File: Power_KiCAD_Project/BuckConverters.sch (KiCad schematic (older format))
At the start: 14 parts

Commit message: added components
added a few components and the correct numbers
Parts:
- removed D? (x2): SBRD10200TR, symbol Device:D_Schottky
- added D5, D6: SBRD10200TR, SBRD10200TR:DPAK228P1005X240-4N, symbol SBRD10200TR:SBRD10200TR
- C21, C22: renamed from C?; symbol 35SVPF82M:35SVPF82M -> Power_KiCAD_Project-rescue:35SVPF82M-35SVPF82M
- C27: renamed from C?; symbol 16SVP330M:16SVP330M -> Power_KiCAD_Project-rescue:16SVP330M-16SVP330M
- C28: renamed from C?; symbol 6SVPC330M:6SVPC330M -> Power_KiCAD_Project-rescue:6SVPC330M-6SVPC330M
- U5, U6: renamed from U?; symbol lm2672m-to-263:LM2672M-TO-263 -> Power_KiCAD_Project-rescue:LM2672M-TO-263-lm2672m-to-263
- gave numbers to parts that had none: 6
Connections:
- net labels added: ground
- net labels removed: GND
- wire segments 46 -> 50
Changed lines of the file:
@@
 $Descr A4 11693 8268
 encoding utf-8
-Sheet 12 12
+Sheet 6 12
 Title "Buck Converter Supply"
 Date "2021-11-29"
@@
 $EndDescr
 $Comp
-L lm2672m-to-263:LM2672M-TO-263 U?
+L Power_KiCAD_Project-rescue:LM2672M-TO-263-lm2672m-to-263 U6
 U 1 1 61A319C7
 P 4900 5200
-F 0 "U?" H 4900 5667 50  0000 C CNN
+F 0 "U6" H 4900 5667 50  0000 C CNN
 F 1 "LM2678SX-3.3/NOPB" H 4900 5576 50  0000 C CNN
 F 2 "Package_TO_SOT_SMD:TO-263-7_TabPin8" H 4950 4850 50  0001 L CIN
@@
 $EndComp
 $Comp
-L Device:C C?
+L Device:C C24
 U 1 1 61A53C7C
 P 4050 5400
-F 0 "C?" H 4200 5400 50  0000 L CNN
+F 0 "C24" H 4200 5400 50  0000 L CNN
 F 1 "C0805C104M5RACTU" V 3900 5000 50  0000 L CNN
 F 2 "Capacitor_SMD:C_0805_2012Metric" H 4088 5250 50  0001 C CNN
@@
 Designed with 3S - 5S lithium pack in mind\nV_IN: 9V - 21V\n\n5A Output
 $Comp
-L 35SVPF82M:35SVPF82M C?
+L Power_KiCAD_Project-rescue:35SVPF82M-35SVPF82M C22
 U 1 1 61A4499B
 P 3400 5250
-F 0 "C?" V 3550 5350 60  0000 L CNN
+F 0 "C22" V 3550 5350 60  0000 L CNN
 F 1 "35SVPF82M" H 3350 5100 60  0000 L CNN
 F 2 "35SVPF82M:35SVPF82M" H 3550 4890 60  0001 C CNN
@@
 	4050 5000 4400 5000
 $Comp
-L Device:C_Small C?
+L Device:C_Small C26
 U 1 1 61A48396
 P 5650 5300
-F 0 "C?" H 5742 5346 50  0000 L CNN
+F 0 "C26" H 5742 5346 50  0000 L CNN
 F 1 "CGA4C2C0G1H103J060AA" H 5700 5250 39  0000 L CNN
 F 2 "Capacitor_SMD:C_0805_2012Metric" H 5650 5300 50  0001 C CNN
@@
 $EndComp
 $Comp
-L pspice:INDUCTOR L?
+L pspice:INDUCTOR L2
 U 1 1 61A496D2
 P 6950 5400
-F 0 "L?" H 6950 5615 50  0000 C CNN
+F 0 "L2" H 6950 5615 50  0000 C CNN
 F 1 "SER2915L-103KL" H 6950 5524 50  0000 C CNN
 F 2 "SER2915L-153KL:SER2915L-153KL" H 6950 5400 50  0001 C CNN
@@
 $EndComp
 $Comp
-L 6SVPC330M:6SVPC330M C?
+L Power_KiCAD_Project-rescue:6SVPC330M-6SVPC330M C28
 U 1 1 61A467E9
 P 7400 5550
-F 0 "C?" V 7500 5750 60  0000 L CNN
+F 0 "C28" V 7500 5750 60  0000 L CNN
 F 1 "6SVPC330M" H 7300 5700 60  0000 L CNN
 F 2 "6SVPC330M:6SVPC330M" H 7550 5190 60  0001 C CNN
@@
 Wire Wire Line
 	7200 5400 7400 5400
-$Comp
-L Device:D_Schottky D?
-U 1 1 61A4C464
-P 6100 5700
-F 0 "D?" V 6054 5780 50  0000 L CNN
-F 1 "SBRD10200TR" H 5850 5600 50  0000 L CNN
-F 2 "" H 6100 5700 50  0001 C CNN
-F 3 "~" H 6100 5700 50  0001 C CNN
-	1    6100 5700
-	0    1    1    0
-$EndComp
-Wire Wire Line
-	6100 6000 6100 5850
-Wire Wire Line
-	6100 6000 7400 6000
-Wire Wire Line
-	6100 5550 6100 5400
-Wire Wire Line
-	6100 5400 6700 5400
+Wire Wire Line
+	6100 6000 6300 6000
 Wire Wire Line
 	7400 5850 7400 6000
@@
 Wire Wire Line
 	5400 5200 5650 5200
-Wire Wire Line
-	5650 5400 6100 5400
 Connection ~ 5650 5400
-Connection ~ 6100 5400
 Wire Wire Line
 	7400 5000 7400 5400
 Wire Wire Line
 	5400 5000 7400 5000
-Connection ~ 6100 6000
-$Comp
-L power:GND #PWR?
-U 1 1 61A58607
-P 4050 5800
-F 0 "#PWR?" H 4050 5550 50  0001 C CNN
-F 1 "GND" H 4055 5627 50  0000 C CNN
-F 2 "" H 4050 5800 50  0001 C CNN
-F 3 "" H 4050 5800 50  0001 C CNN
-	1    4050 5800
-	1    0    0    -1
-$EndComp
-$Comp
-L power:GND #PWR?
-U 1 1 61A58BE6
-P 6100 6000
-F 0 "#PWR?" H 6100 5750 50  0001 C CNN
-F 1 "GND" H 6105 5827 50  0000 C CNN
-F 2 "" H 6100 6000 50  0001 C CNN
-F 3 "" H 6100 6000 50  0001 C CNN
-	1    6100 6000
-	1    0    0    -1
-$EndComp
 NoConn ~ 4400 5400
 Wire Notes Line
@@
 3.3V Buck Converter
 $Comp
-L lm2672m-to-263:LM2672M-TO-263 U?
+L Power_KiCAD_Project-rescue:LM2672M-TO-263-lm2672m-to-263 U5
 U 1 1 61A7F0DE
 P 4900 2850
-F 0 "U?" H 4900 3317 50  0000 C CNN
+F 0 "U5" H 4900 3317 50  0000 C CNN
 F 1 "LM2678SX-5.0/NOPB" H 4900 3226 50  0000 C CNN
 F 2 "Package_TO_SOT_SMD:TO-263-7_TabPin8" H 4950 2500 50  0001 L CIN
@@
 $EndComp
 $Comp
-L Device:C C?
+L Device:C C23
 U 1 1 61A7F0E5
 P 4050 3050
-F 0 "C?" H 4200 3050 50  0000 L CNN
+F 0 "C23" H 4200 3050 50  0000 L CNN
 F 1 "C0805C104M5RACTU" V 3900 2650 50  0000 L CNN
 F 2 "Capacitor_SMD:C_0805_2012Metric" H 4088 2900 50  0001 C CNN
@@
 $EndComp
 Wire Wire Line
-	3400 2650 3400 2900
-Wire Wire Line
 	3400 3450 3400 3200
 Wire Wire Line
 	4900 3450 4900 3250
-Wire Wire Line
-	3400 2650 3250 2650
-Connection ~ 3400 2650
 Text HLabel 3250 2650 0    50   Input ~ 0
 V_IN
 $Comp
-L 35SVPF82M:35SVPF82M C?
+L Power_KiCAD_Project-rescue:35SVPF82M-35SVPF82M C21
 U 1 1 61A7F0F2
 P 3400 2900
-F 0 "C?" V 3550 3000 60  0000 L CNN
+F 0 "C21" V 3550 3000 60  0000 L CNN
 F 1 "35SVPF82M" H 3350 2750 60  0000 L CNN
 F 2 "35SVPF82M:35SVPF82M" H 3550 2540 60  0001 C CNN
@@
 	3400 3450 4050 3450
 Wire Wire Line
-	3400 2650 4050 2650
-Wire Wire Line
 	4050 3200 4050 3450
 Connection ~ 4050 3450
@@
 	4050 2650 4400 2650
 $Comp
-L Device:C_Small C?
+L Device:C_Small C25
 U 1 1 61A7F101
 P 5650 2950
-F 0 "C?" H 5742 2996 50  0000 L CNN
+F 0 "C25" H 5742 2996 50  0000 L CNN
 F 1 "CGA4C2C0G1H103J060AA" H 5700 2900 39  0000 L CNN
 F 2 "Capacitor_SMD:C_0805_2012Metric" H 5650 2950 50  0001 C CNN
@@
 $EndComp
 $Comp
-L pspice:INDUCTOR L?
+L pspice:INDUCTOR L1
 U 1 1 61A7F108
 P 6950 3050
-F 0 "L?" H 6950 3265 50  0000 C CNN
+F 0 "L1" H 6950 3265 50  0000 C CNN
 F 1 "MSS1210-153MEB" H 6950 3174 50  0000 C CNN
 F 2 "MSS1210-153MEB:INDPM120120X1020N" H 6950 3050 50  0001 C CNN
@@
 Wire Wire Line
 	7200 3050 7400 3050
-$Comp
-L Device:D_Schottky D?
-U 1 1 61A7F115
-P 6100 3350
-F 0 "D?" V 6054 3430 50  0000 L CNN
-F 1 "SBRD10200TR" H 5850 3250 50  0000 L CNN
-F 2 "" H 6100 3350 50  0001 C CNN
-F 3 "~" H 6100 3350 50  0001 C CNN
-	1    6100 3350
-	0    1    1    0
-$EndComp
-Wire Wire Line
-	6100 3650 6100 3500
-Wire Wire Line
-	6100 3650 7400 3650
 Wire Wire Line
 	6100 3200 6100 3050
@@
 Wire Wire Line
 	5400 2650 7400 2650
-Connection ~ 6100 3650
-$Comp
-L power:GND #PWR?
-U 1 1 61A7F12C
-P 4050 3450
-F 0 "#PWR?" H 4050 3200 50  0001 C CNN
-F 1 "GND" H 4055 3277 50  0000 C CNN
-F 2 "" H 4050 3450 50  0001 C CNN
-F 3 "" H 4050 3450 50  0001 C CNN
-	1    4050 3450
-	1    0    0    -1
-$EndComp
-$Comp
-L power:GND #PWR?
-U 1 1 61A7F132
-P 6100 3650
-F 0 "#PWR?" H 6100 3400 50  0001 C CNN
-F 1 "GND" H 6105 3477 50  0000 C CNN
-F 2 "" H 6100 3650 50  0001 C CNN
-F 3 "" H 6100 3650 50  0001 C CNN
-	1    6100 3650
-	1    0    0    -1
-$EndComp
 NoConn ~ 4400 3050
 Wire Notes Line
@@
 5V Buck Converter
 $Comp
-L 16SVP330M:16SVP330M C?
+L Power_KiCAD_Project-rescue:16SVP330M-16SVP330M C?
 U 1 1 61A47D3A
 P 7400 3200
-F 0 "C?" V 7497 3305 60  0000 L CNN
+AR Path="/61A47D3A" Ref="C?"  Part="1"
+AR Path="/61A48488/61A47D3A" Ref="C27"  Part="1"
+F 0 "C27" V 7497 3305 60  0000 L CNN
 F 1 "16SVP330M" V 7603 3305 60  0000 L CNN
 F 2 "PCAP_SVP_F12_PAN" H 7550 2840 60  0001 C CNN
@@
 Wire Wire Line
 	3400 5800 3400 5550
+Text HLabel 4050 3450 3    50   Input ~ 0
+ground
+Text HLabel 6000 3650 0    50   Input ~ 0
+ground
+Text HLabel 6100 6000 0    50   Input ~ 0
+ground
+Text HLabel 4050 5800 3    50   Input ~ 0
+ground
+$Comp
+L SBRD10200TR:SBRD10200TR D5
+U 1 1 61A8FF3C
+P 6100 3400
+F 0 "D5" H 6276 3441 50  0000 L CNN
+F 1 "SBRD10200TR" H 6276 3350 50  0000 L CNN
+F 2 "SBRD10200TR:DPAK228P1005X240-4N" H 6100 3400 50  0001 L BNN
+F 3 "" H 6100 3400 50  0001 L BNN
+F 4 "SBRD10200TR" H 6100 3400 50  0001 L BNN "MP"
+F 5 "1655-1939-1-ND" H 6100 3400 50  0001 L BNN "Digi-Key_Part_Number"
+F 6 "TO-252-3 SMC" H 6100 3400 50  0001 L BNN "Package"
+F 7 "Diode Schottky 200 V 10A Surface Mount DPAK" H 6100 3400 50  0001 L BNN "Description"
+F 8 "SMC Diode" H 6100 3400 50  0001 L BNN "MF"
+	1    6100 3400
+	1    0    0    -1
+$EndComp
+$Comp
+L SBRD10200TR:SBRD10200TR D6
+U 1 1 61A94D59
+P 6200 5600
+F 0 "D6" H 6376 5641 50  0000 L CNN
+F 1 "SBRD10200TR" H 6376 5550 50  0000 L CNN
+F 2 "SBRD10200TR:DPAK228P1005X240-4N" H 6200 5600 50  0001 L BNN
+F 3 "" H 6200 5600 50  0001 L BNN
+F 4 "SBRD10200TR" H 6200 5600 50  0001 L BNN "MP"
+F 5 "1655-1939-1-ND" H 6200 5600 50  0001 L BNN "Digi-Key_Part_Number"
+F 6 "TO-252-3 SMC" H 6200 5600 50  0001 L BNN "Package"
+F 7 "Diode Schottky 200 V 10A Surface Mount DPAK" H 6200 5600 50  0001 L BNN "Description"
+F 8 "SMC Diode" H 6200 5600 50  0001 L BNN "MF"
+	1    6200 5600
+	1    0    0    -1
+$EndComp
+Wire Wire Line
+	5650 5400 6200 5400
+Connection ~ 6200 5400
+Wire Wire Line
+	6200 5400 6700 5400
+Wire Wire Line
+	6300 5800 6300 6000
+Connection ~ 6300 6000
+Wire Wire Line
+	6300 6000 7400 6000
+Wire Wire Line
+	6100 5800 6100 6000
+Wire Wire Line
+	6000 3650 6200 3650
+Wire Wire Line
+	6000 3600 6000 3610
+Connection ~ 6000 3610
+Wire Wire Line
+	6000 3610 6000 3650
+Wire Wire Line
+	6200 3600 6200 3650
+Connection ~ 6200 3650
+Wire Wire Line
+	6200 3650 7400 3650
+Wire Wire Line
+	3250 2650 3400 2650
+Wire Wire Line
+	3400 2900 3400 2650
+Connection ~ 3400 2650
+Wire Wire Line
+	3400 2650 4050 2650
 $EndSCHEMATC

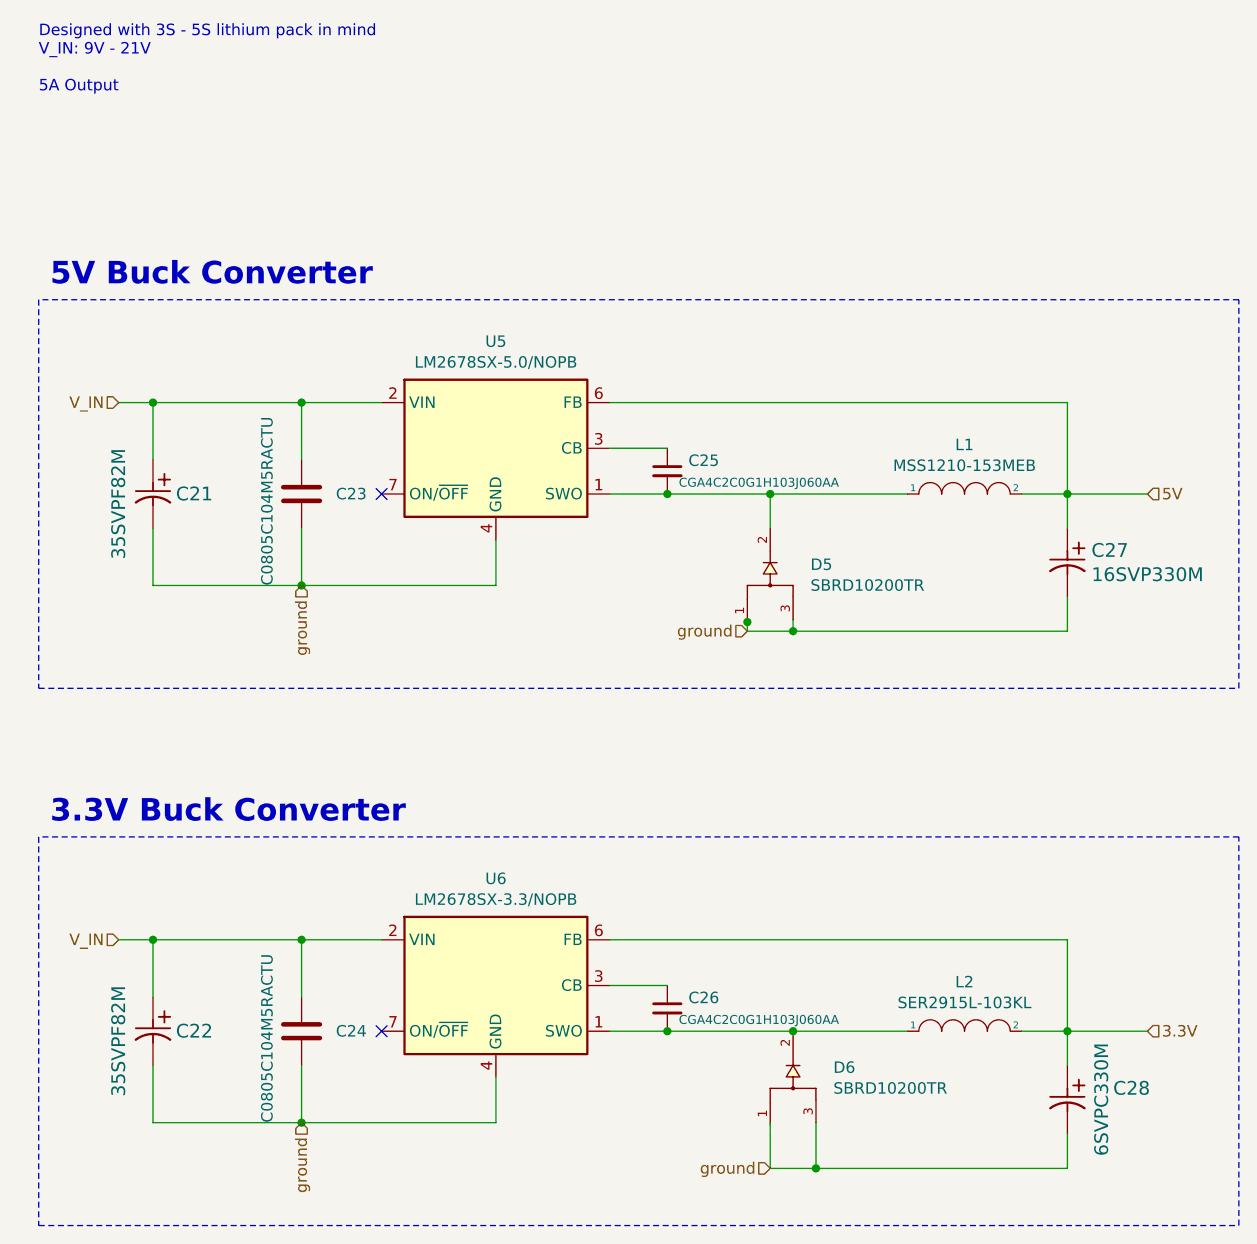
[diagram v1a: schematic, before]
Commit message: pcb finished
pcb is done. 3am kicad be like
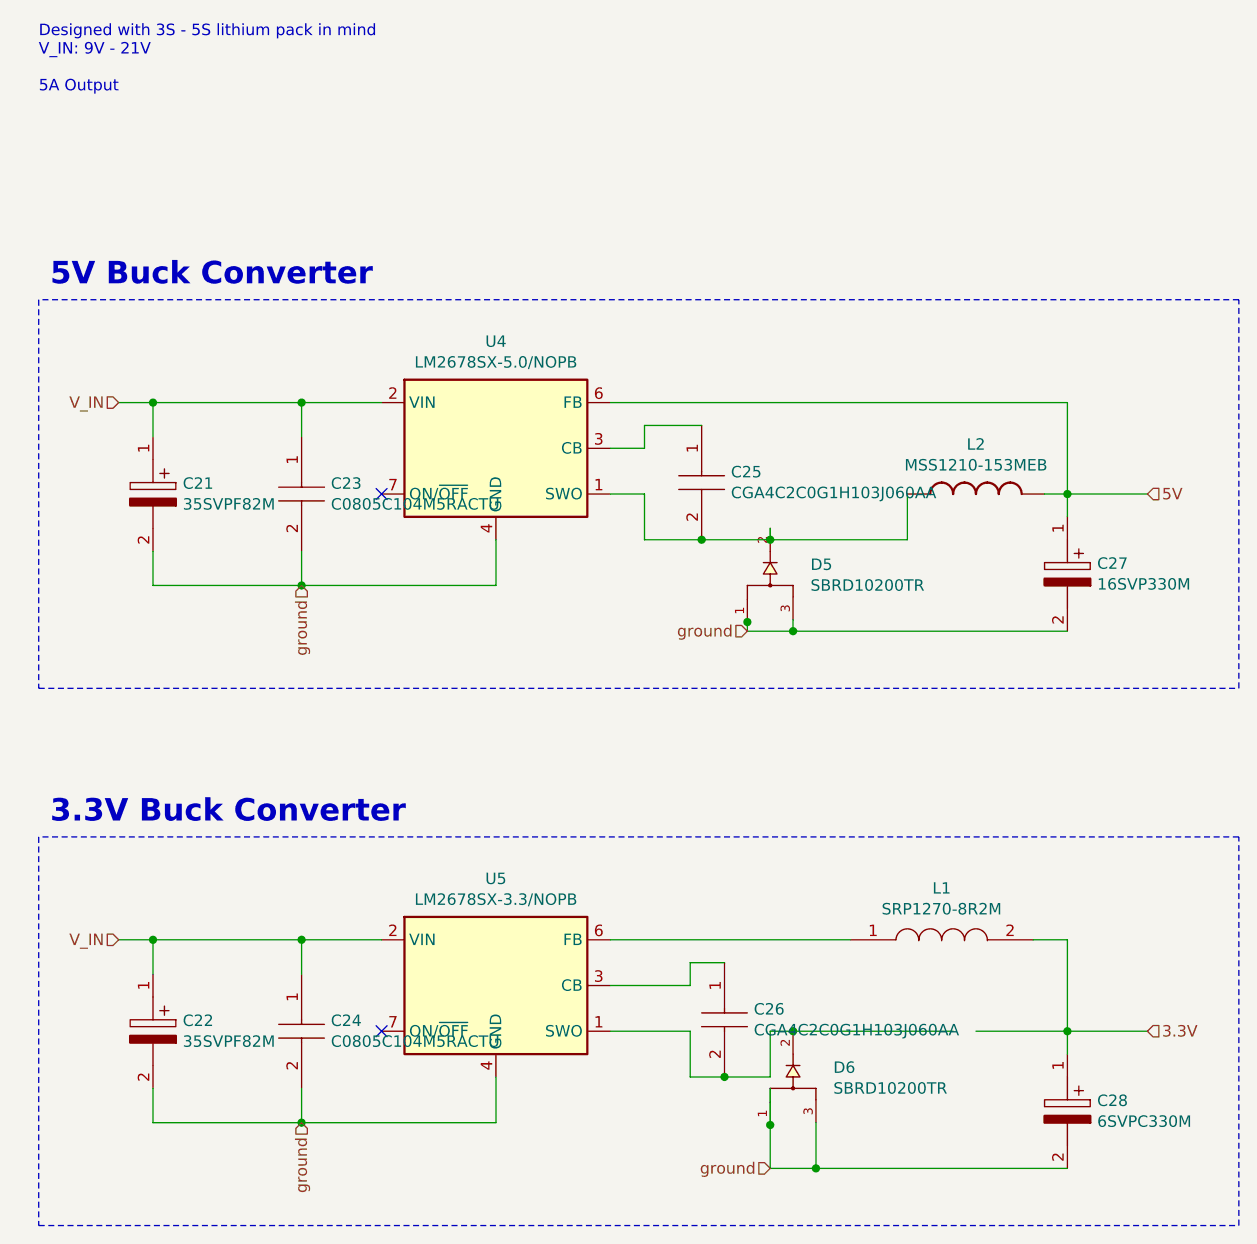
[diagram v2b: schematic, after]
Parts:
- removed C21, C22: 35SVPF82M, 35SVPF82M:35SVPF82M, symbol Power_KiCAD_Project-rescue:35SVPF82M-35SVPF82M
- removed C23, C24: C0805C104M5RACTU, Capacitor_SMD:C_0805_2012Metric, symbol Device:C
- removed C25, C26: CGA4C2C0G1H103J060AA, Capacitor_SMD:C_0805_2012Metric, symbol Device:C_Small
- removed C27: 16SVP330M, PCAP_SVP_F12_PAN, symbol Power_KiCAD_Project-rescue:16SVP330M-16SVP330M
- removed C28: 6SVPC330M, 6SVPC330M:6SVPC330M, symbol Power_KiCAD_Project-rescue:6SVPC330M-6SVPC330M
- removed L1: MSS1210-153MEB, MSS1210-153MEB:INDPM120120X1020N, symbol pspice:INDUCTOR
- removed L2: SER2915L-103KL, SER2915L-153KL:SER2915L-153KL, symbol pspice:INDUCTOR
- added C21, C22: 35SVPF82M, SamacSys_Parts:16SVPT560M, symbol SamacSys_Parts:35SVPF82M
- added C23, C24: C0805C104M5RACTU, SamacSys_Parts:CAPC2012X88N, symbol SamacSys_Parts:C0805C104M5RACTU
- added C25, C26: CGA4C2C0G1H103J060AA, SamacSys_Parts:CAPC2012X75N, symbol SamacSys_Parts:CGA4C2C0G1H103J060AA
- added C27: 16SVP330M, SamacSys_Parts:16SVF1000M, symbol SamacSys_Parts:16SVP330M
- added C28: 6SVPC330M, SamacSys_Parts:16SVF180M, symbol SamacSys_Parts:6SVPC330M
- added L1: SRP1270-8R2M, SamacSys_Parts:INDPM137129X700N, symbol SamacSys_Parts:SRP1270-8R2M
- added L2: MSS1210-153MEB, MSS1210-153MEB:IND_MSS1210-153MEB, symbol MSS1210-153MEB:MSS1210-153MEB
- renumbered U5 to U4, U6 to U5
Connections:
- wire segments 50 -> 61
